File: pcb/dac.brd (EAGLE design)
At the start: 69.5 x 58.4 mm, 16 parts, among them Q1 2N7000, U1 PIC16F1773-I/SP

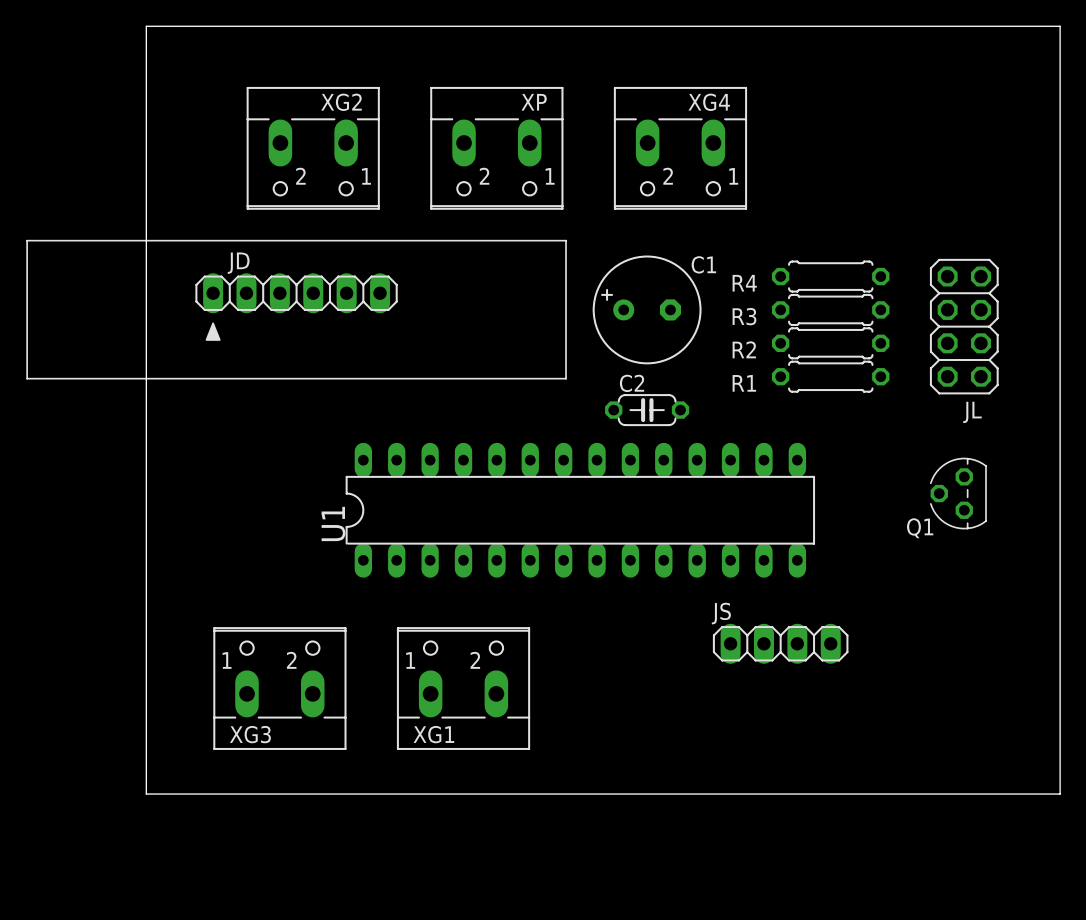
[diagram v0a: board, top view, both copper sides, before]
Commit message: Protoboard layout & routing
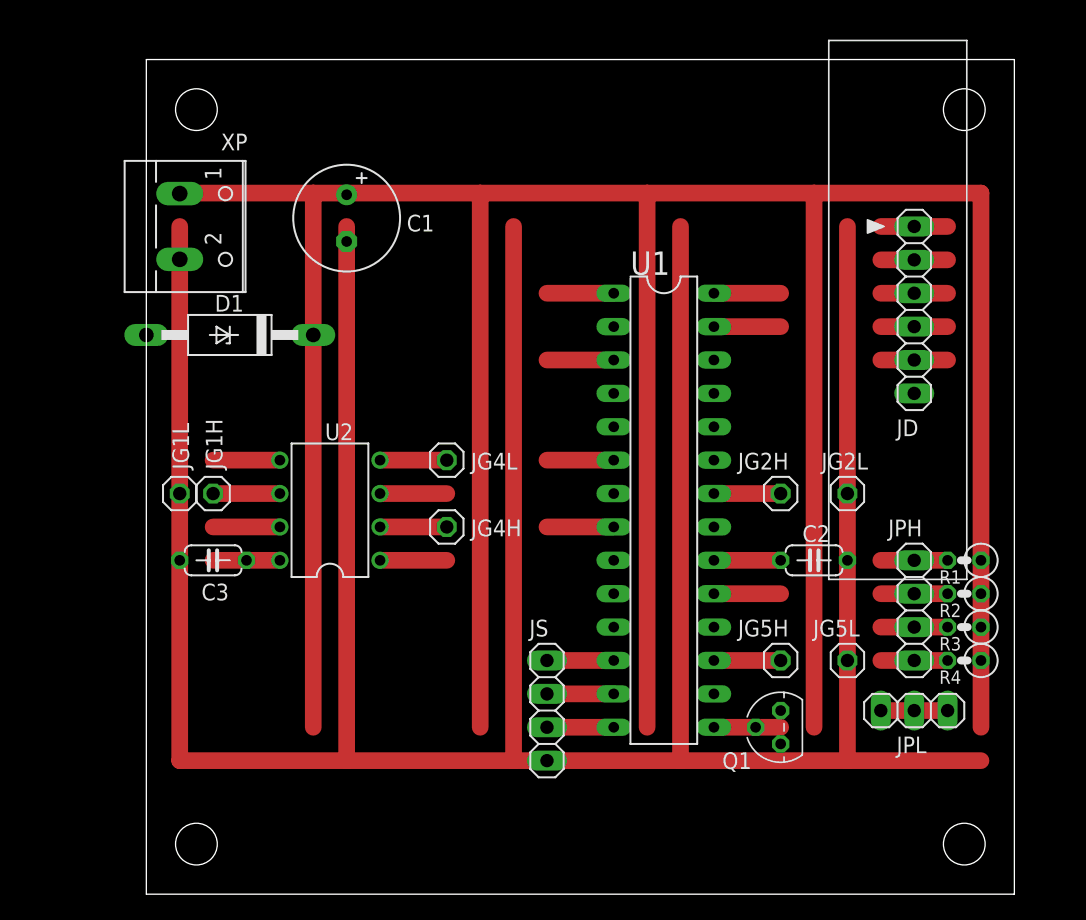
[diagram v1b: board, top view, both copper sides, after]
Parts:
- removed JL: (no value), pinhead:2X04
- removed XG1, XG2, XG3, XG4: (no value), con-wago-500:W237-102
- added C3: 2.2uF, rcl:C050-024X044
- added D1: SA5.0A, diode:P1Z12
- added JG1H, JG1L, JG2H, JG2L, JG4H, JG4L, JG5H, JG5L: (no value), pinhead:1X01
- added JPH: (no value), pinhead:1X04
- added JPL: (no value), pinhead:1X03
- added U2: MCP6002-I/P, linear:DIL08
- R1, R2, R3, R4: device rcl:0207/7 -> rcl:0207/2V
- moved JD 47.0 mm to (58.4, 36.8), turned to 270 degrees
- moved R4 30.9 mm to (62.2, 10.2)
- moved R3 26.2 mm to (62.2, 12.7)
- moved C1 23.9 mm to (15.2, 43.8), turned to 270 degrees
- moved XP 23.4 mm to (3.81, 43.2), turned to 270 degrees
- moved Q1 22.6 mm to (48.3, 5.08)
- moved R2 21.6 mm to (62.2, 15.2)
- moved JS 18.5 mm to (30.5, 6.35), turned to 270 degrees
- moved R1 17.3 mm to (62.2, 17.8)
- moved C2 17.1 mm to (50.8, 17.8)
- moved U1 6.35 mm to (39.4, 21.6), turned to 270 degrees
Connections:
- removed net N$1: JL.1, JL.3, JL.5, JL.7, Q1.3
- new net DAC1_UNBUF: U1.3, U2.5
- new net FADE_L: JPL.1, JPL.2, JPL.3, Q1.3
- net +5V: now also C3.1, D1.C, R1.1, R2.1, R3.1, R4.1, U2.8; no longer R1.2, R2.2, R3.2, R4.2
- net DAC1: now also JG1H.1, U2.6, U2.7; no longer U1.3, XG1.1
- net DAC2: now also JG2H.1; no longer XG2.1
- net DAC4: now also JG4H.1, U2.1, U2.2; no longer XG3.1
- net DAC4_UNBUF: now also U2.3
- net DAC5: now also JG5H.1; no longer XG4.1
- net GND: now also C3.2, D1.A, JG1L.1, JG2L.1, JG4L.1, JG5L.1, U2.4; no longer XG1.2, XG2.2, XG3.2, XG4.2
- net LED1: now also JPH.1, R1.2; no longer JL.2, R1.1
- net LED2: now also JPH.2, R2.2; no longer JL.4, R2.1
- net LED3: now also JPH.3, R3.2; no longer JL.6, R3.1
- net LED4: now also JPH.4, R4.2; no longer JL.8, R4.1
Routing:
- net GND: track 0.00 -> 284.5 mm
- net +5V: track 0.00 -> 279.4 mm
- net DAC1_UNBUF: track 0.00 -> 10.2 mm
- net DAC4_UNBUF: track 0.00 -> 10.2 mm
- net DAC1: track 0.00 -> 10.2 mm
- net !MCLR: track 0.00 -> 10.2 mm
- net PGD: track 0.00 -> 10.2 mm
- net PGC: track 0.00 -> 10.2 mm
- net DAC4: track 0.00 -> 10.2 mm
- net SCLK: track 0.00 -> 5.08 mm
- net MOSI: track 0.00 -> 5.08 mm
- net MISO: track 0.00 -> 5.08 mm
- net LED4: track 0.00 -> 5.08 mm
- net LED3: track 0.00 -> 5.08 mm
- net LED2: track 0.00 -> 5.08 mm
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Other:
- board size 69.5 x 58.4 mm -> 66 x 63.5 mm
- board text added: "www.PROTO-ADVANTAGE.com SBB1605-1"
